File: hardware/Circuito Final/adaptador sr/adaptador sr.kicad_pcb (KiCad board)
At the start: 2 copper layers, 9.3 x 20.5 mm, 1 part, among them U2 74HC595

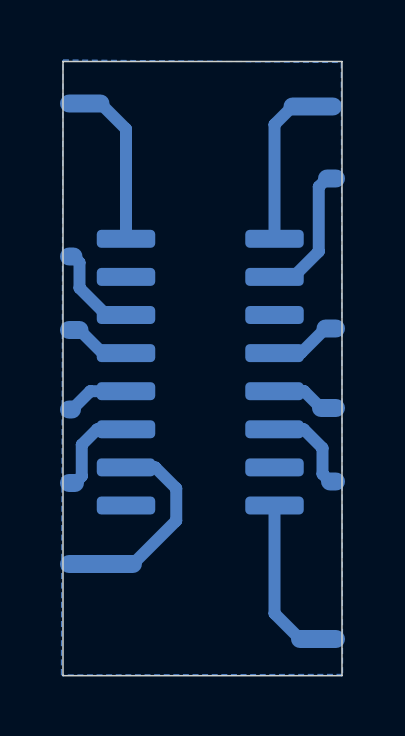
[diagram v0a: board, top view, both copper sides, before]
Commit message: pruebas del shift register
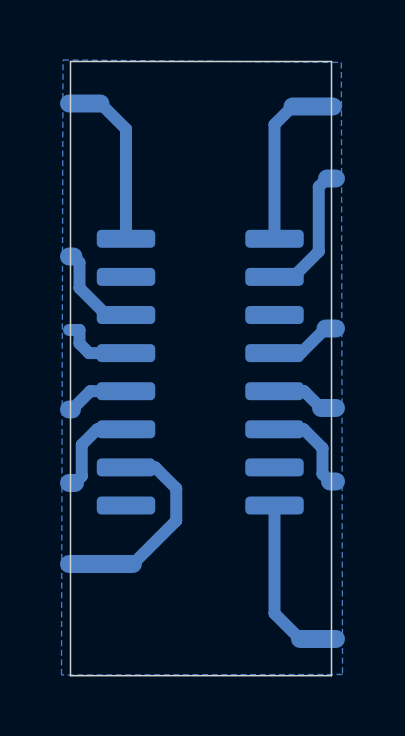
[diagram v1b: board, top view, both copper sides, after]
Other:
- board size 9.3 x 20.5 mm -> 8.7 x 20.5 mm
